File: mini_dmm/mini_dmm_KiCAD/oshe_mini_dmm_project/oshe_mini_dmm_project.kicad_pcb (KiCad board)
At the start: 4 copper layers, 54 x 86 mm, 45 parts, among them J1 FTDI Basic, J2 ICSP, J3 DISPLAY, J4 TEST LEAD CONNECTIONS, SW1 PTS526 SK15 SMTR2 LFS, SW2 PTS526 SK15 SMTR2 LFS, SW3 SW_DPDT_x2, U1 LM324, U2 ATmega328P-A, U3 BU91796FS-ME2, U4 LM2664M6, Y1 16MHz

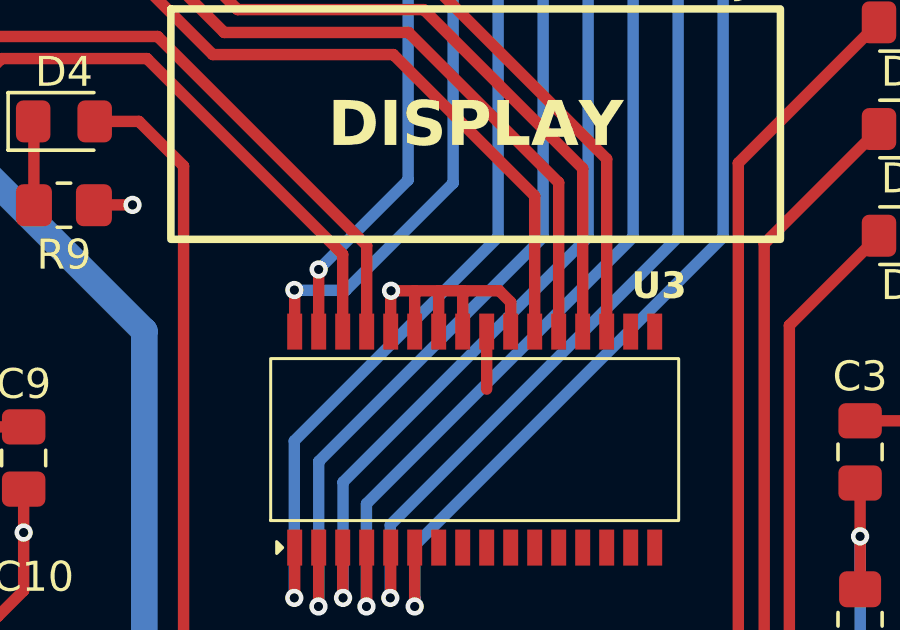
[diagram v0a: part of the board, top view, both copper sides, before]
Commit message: Exported final board
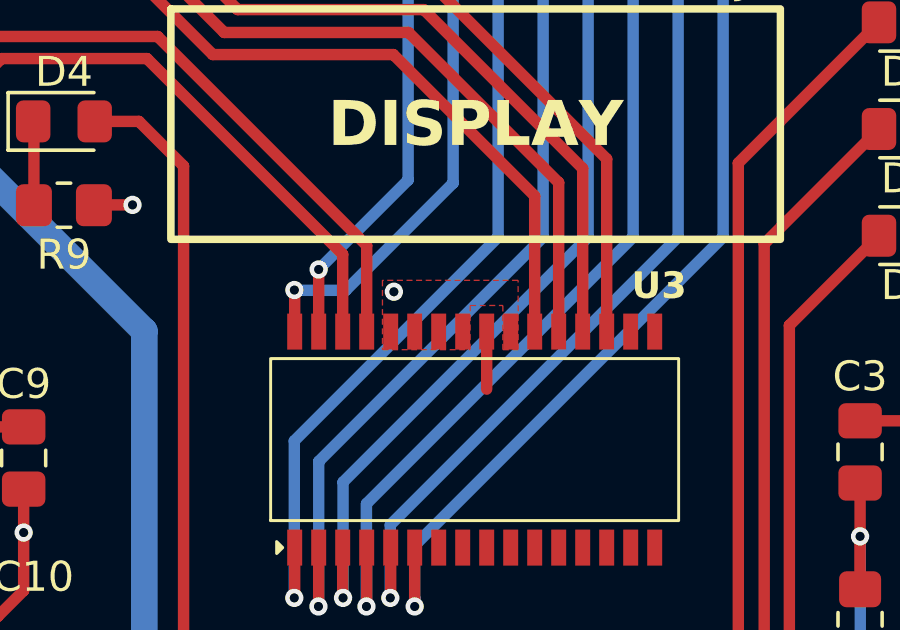
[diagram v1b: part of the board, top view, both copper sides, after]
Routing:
- net GND: track 89.7 -> 79.1 mm
- added copper zone on F.Cu, net GND
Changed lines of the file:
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@@
 			(size 1 1)
 			(drill 1)
-			(layers "F&B.Cu" "*.Mask")
+			(layers "*.Cu" "*.Mask")
 		)
 		(pad "" np_thru_hole circle
@@
 			(size 1 1)
 			(drill 1)
-			(layers "F&B.Cu" "*.Mask")
+			(layers "*.Cu" "*.Mask")
 		)
 		(pad "1" smd rect
@@
 	)
 	(segment
-		(start 150.3758 76.727)
-		(end 150.3754 76.7266)
-		(width 0.381)
-		(layer "F.Cu")
-		(net 2)
-	)
-	(segment
-		(start 151.1758 76.739)
-		(end 151.1882 76.7266)
-		(width 0.381)
-		(layer "F.Cu")
-		(net 2)
-	)
-	(segment
 		(start 146.1421 126.5936)
 		(end 146.1513 126.6028)
@@
 	)
 	(segment
-		(start 149.5758 76.7388)
-		(end 149.588 76.7266)
-		(width 0.381)
-		(layer "F.Cu")
-		(net 2)
-	)
-	(segment
 		(start 132.6681 115.4684)
 		(end 132.6681 115.2945)
@@
 	)
 	(segment
-		(start 151.1758 78.0864)
-		(end 151.1758 76.739)
-		(width 0.381)
-		(layer "F.Cu")
-		(net 2)
-	)
-	(segment
 		(start 137.405 113.3602)
 		(end 134.62 113.3602)
@@
 	)
 	(segment
-		(start 153.197 76.7266)
-		(end 151.9756 76.7266)
-		(width 0.381)
-		(layer "F.Cu")
-		(net 2)
-	)
-	(segment
 		(start 174.7468 71.3232)
 		(end 174.736 71.334)
@@
 	)
 	(segment
-		(start 153.5758 77.1054)
-		(end 153.197 76.7266)
-		(width 0.381)
-		(layer "F.Cu")
-		(net 2)
-	)
-	(segment
 		(start 174.7308 67.7672)
 		(end 174.72 67.778)
@@
 	)
 	(segment
-		(start 150.3754 76.7266)
-		(end 149.588 76.7266)
-		(width 0.381)
-		(layer "F.Cu")
-		(net 2)
-	)
-	(segment
 		(start 146.1513 126.6028)
 		(end 146.1513 124.6083)
@@
 	)
 	(segment
-		(start 151.9758 76.7268)
-		(end 151.9756 76.7266)
-		(width 0.381)
-		(layer "F.Cu")
-		(net 2)
-	)
-	(segment
 		(start 156.8704 98.3234)
 		(end 155.702 99.4918)
@@
 	)
 	(segment
-		(start 150.3758 78.0864)
-		(end 150.3758 76.727)
-		(width 0.381)
-		(layer "F.Cu")
-		(net 2)
-	)
-	(segment
 		(start 134.62 113.3602)
 		(end 132.6681 115.3121)
@@
 	)
 	(segment
-		(start 151.1882 76.7266)
-		(end 150.3754 76.7266)
-		(width 0.381)
-		(layer "F.Cu")
-		(net 2)
-	)
-	(segment
 		(start 131.2672 113.8936)
 		(end 131.2672 112.98555)
@@
 	)
 	(segment
-		(start 151.9756 76.7266)
-		(end 151.1882 76.7266)
-		(width 0.381)
-		(layer "F.Cu")
-		(net 2)
-	)
-	(segment
-		(start 151.9758 78.0864)
-		(end 151.9758 76.7268)
-		(width 0.381)
-		(layer "F.Cu")
-		(net 2)
-	)
-	(segment
 		(start 153.1874 89.0524)
 		(end 156.8704 92.7354)
@@
 	)
 	(segment
-		(start 149.5758 78.0864)
-		(end 149.5758 76.7388)
-		(width 0.381)
-		(layer "F.Cu")
-		(net 2)
-	)
-	(segment
 		(start 133.1763 126.63815)
 		(end 133.1662 126.62805)
@@
 	)
 	(segment
-		(start 153.5758 78.0864)
-		(end 153.5758 77.1054)
-		(width 0.381)
-		(layer "F.Cu")
-		(net 2)
-	)
-	(segment
 		(start 155.702 99.4918)
 		(end 155.47975 99.4918)
@@
 	)
 	(via
-		(at 149.588 76.7266)
+		(at 149.6822 76.7588)
 		(size 0.6096)
 		(drill 0.3048)
@@
 	)
 	(zone
+		(net 2)
+		(net_name "GND")
+		(layer "F.Cu")
+		(hatch edge 0.5)
+		(priority 3)
+		(connect_pads yes
+			(clearance 0.254)
+		)
+		(min_thickness 0.25)
+		(filled_areas_thickness no)
+		(fill yes
+			(thermal_gap 0.5)
+			(thermal_bridge_width 0.5)
+		)
+		(polygon
+			(pts
+				(xy 149.3012 78.6892) (xy 152.2222 78.6892) (xy 152.2222 77.216) (xy 153.3144 77.216) (xy 153.3144 78.6892)
+				(xy 153.8224 78.6892) (xy 153.8224 76.3778) (xy 149.3012 76.3778)
+			)
+		)
+	)
+	(zone
